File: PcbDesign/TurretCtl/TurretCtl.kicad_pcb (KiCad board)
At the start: 4 copper layers, 69.6 x 54.4 mm, 28 parts, among them J1 FLIR, J2 Stepper1, J3 Stepper2, J4 PWR

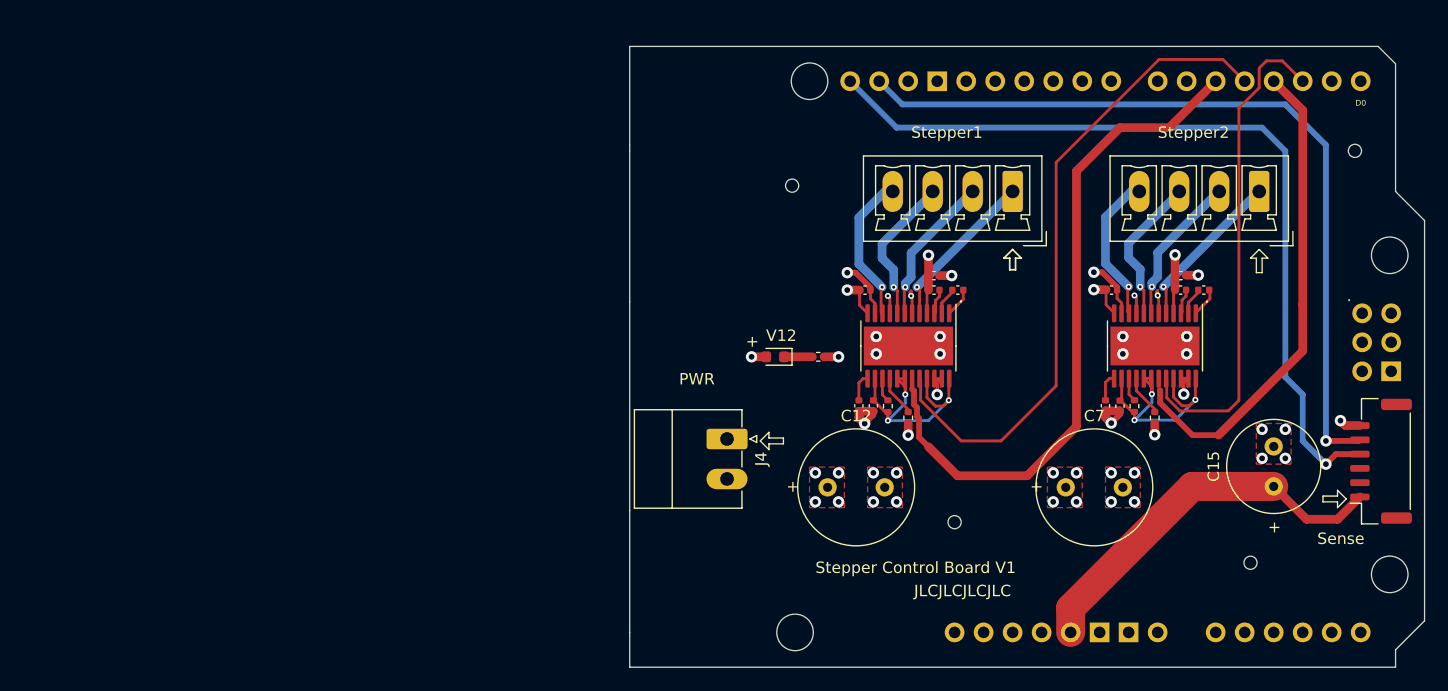
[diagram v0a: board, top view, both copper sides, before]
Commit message: Stepper Control Board V2
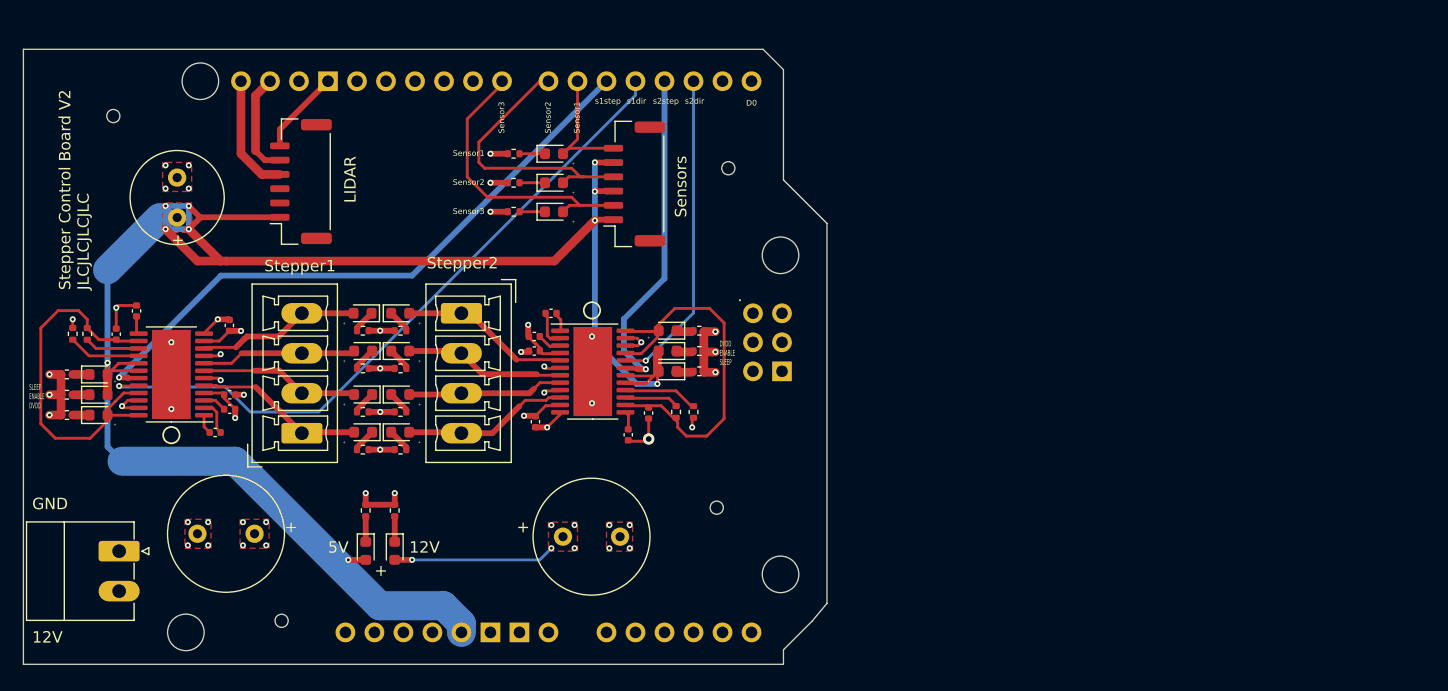
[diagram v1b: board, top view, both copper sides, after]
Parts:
- added D10: LED, LED_SMD:LED_0603_1608Metric, F.Cu at (29.2, 92.7)
- added D11: LED, LED_SMD:LED_0603_1608Metric, F.Cu at (79.0, 85.3)
- added D12: LED, LED_SMD:LED_0603_1608Metric, F.Cu at (29.2, 89.2)
- added D13: LED, LED_SMD:LED_0603_1608Metric, F.Cu at (79.0, 88.9)
- added D14: LED, LED_SMD:LED_0603_1608Metric, F.Cu at (52.6, 104.6)
- added D15: LED, LED_SMD:LED_0603_1608Metric, F.Cu at (69.1, 69.8)
- added D16: LED, LED_SMD:LED_0603_1608Metric, F.Cu at (29.2, 91.0)
- added D17: LED, LED_SMD:LED_0603_1608Metric, F.Cu at (79.0, 87.1)
- added D18: LED, LED_SMD:LED_0603_1608Metric, F.Cu at (69.1, 72.4)
- added D19: LED, LED_SMD:LED_0603_1608Metric, F.Cu at (69.1, 74.9)
- added D2: LED, LED_SMD:LED_0603_1608Metric, F.Cu at (52.3, 83.8)
- added D3: LED, LED_SMD:LED_0603_1608Metric, F.Cu at (55.6, 94.2)
- added D4: LED, LED_SMD:LED_0603_1608Metric, F.Cu at (52.3, 87.1)
- added D5: LED, LED_SMD:LED_0603_1608Metric, F.Cu at (55.6, 90.9)
- added D6: LED, LED_SMD:LED_0603_1608Metric, F.Cu at (52.3, 90.9)
- added D7: LED, LED_SMD:LED_0603_1608Metric, F.Cu at (55.6, 87.1)
- added D8: LED, LED_SMD:LED_0603_1608Metric, F.Cu at (52.3, 94.2)
- added D9: LED, LED_SMD:LED_0603_1608Metric, F.Cu at (55.6, 83.8)
- added J5: Sensors, Connector_JST:JST_GH_SM06B-GHS-TB_1x06-1MP_P1.25mm_Horizontal, F.Cu at (76.1, 72.5)
- added R10: 330, Resistor_SMD:R_0402_1005Metric, F.Cu at (52.3, 92.5)
- added R11: 330, Resistor_SMD:R_0402_1005Metric, F.Cu at (55.6, 88.6)
- added R12: 330, Resistor_SMD:R_0402_1005Metric, F.Cu at (52.3, 95.8)
- added R13: 330, Resistor_SMD:R_0402_1005Metric, F.Cu at (55.6, 85.3)
- added R14: 330, Resistor_SMD:R_0402_1005Metric, F.Cu at (26.4, 92.7)
- added R15: 330, Resistor_SMD:R_0402_1005Metric, F.Cu at (81.8, 85.3)
- added R16: 330, Resistor_SMD:R_0402_1005Metric, F.Cu at (26.4, 89.2)
- added R17: 330, Resistor_SMD:R_0402_1005Metric, F.Cu at (81.8, 88.9)
- added R18: 330, Resistor_SMD:R_0402_1005Metric, F.Cu at (52.6, 101.1)
- added R19: 330, Resistor_SMD:R_0402_1005Metric, F.Cu at (65.5, 69.8)
- added R20: 330, Resistor_SMD:R_0402_1005Metric, F.Cu at (26.4, 91.0)
- added R21: 330, Resistor_SMD:R_0402_1005Metric, F.Cu at (81.8, 87.1)
- added R22: 330, Resistor_SMD:R_0402_1005Metric, F.Cu at (65.5, 72.4)
- added R23: 330, Resistor_SMD:R_0402_1005Metric, F.Cu at (65.5, 74.9)
- added R6: 330, Resistor_SMD:R_0402_1005Metric, F.Cu at (52.3, 85.3)
- added R7: 330, Resistor_SMD:R_0402_1005Metric, F.Cu at (55.6, 95.8)
- added R8: 330, Resistor_SMD:R_0402_1005Metric, F.Cu at (52.3, 88.6)
- added R9: 330, Resistor_SMD:R_0402_1005Metric, F.Cu at (55.6, 92.5)
- R5: value 290 -> 330
- moved C15 98.9 mm to (36.1, 75.4)
- moved J1 97.7 mm to (46.9, 72.3)
- moved R1 73.5 mm to (26.9, 85.6), turned to 90 degrees
- moved C7 71.1 mm to (42.8, 103.1), turned to 180 degrees
- moved J3 70.7 mm to (61.0, 83.8), turned to -90 degrees
- moved R2 70.4 mm to (28.2, 85.6), turned to -90 degrees
- moved C8 66.6 mm to (30.7, 85.6), turned to 90 degrees
- moved C3 66.2 mm to (39.4, 94.3), turned to 180 degrees
- moved J2 65.7 mm to (47.0, 94.3), turned to 90 degrees
- moved U2 64.6 mm to (35.6, 89.2), turned to 180 degrees
- moved C9 63.8 mm to (32.5, 83.6), turned to 90 degrees
- moved C4 62.5 mm to (40.7, 92.2), turned to 180 degrees
- moved C6 62.5 mm to (40.7, 91.0)
- moved C11 57.9 mm to (67.4, 93.3), turned to -90 degrees
- moved C1 57.2 mm to (68.8, 83.8)
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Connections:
- U1 pad 17: /Stepper2/DVDD -> +5V
- U1 pad 18: /Stepper2/DVDD -> +5V
- U1 pad 25: GND -> (no net)
- U2 pad 17: /Stepper1/DVDD -> +5V
- U2 pad 18: /Stepper1/DVDD -> +5V
- U2 pad 25: GND -> (no net)
- XA1 pad D6: unconnected-(XA1-PadD6) -> D6
- XA1 pad D7: unconnected-(XA1-PadD7) -> D7
- XA1 pad D8: unconnected-(XA1-PadD8) -> D8
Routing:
- net +5V: track 33.9 -> 176.6 mm, vias 0 -> 12
- net SCL: track 72.9 -> 10.5 mm, vias 1 -> 0
- net SDA: track 70.4 -> 9.09 mm, vias 1 -> 0
- net GND: track 36.9 -> 67.2 mm, vias 36 -> 41
- net D8: track 0.00 -> 25.2 mm
- net D7: track 0.00 -> 24.4 mm
- net S2_DIR: track 43.5 -> 28.0 mm, vias 0 -> 1
- net S2_STEP: track 42.5 -> 30.4 mm, vias 0 -> 1
- net D6: track 0.00 -> 11.5 mm
- net /Stepper1/DVDD: track 23.7 -> 33.2 mm, vias 3 -> 0
- net /Stepper2/DVDD: track 23.7 -> 33.0 mm, vias 3 -> 0
- net +12V: track 21.5 -> 30.2 mm
- net S1_STEP: track 59.2 -> 56.0 mm, vias 0 -> 1
- net /Stepper2/RREF: track 3.58 -> 6.36 mm
- net /Stepper1/RREF: track 3.58 -> 6.36 mm
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- added copper zone on B.Cu, net +5V
- added copper zone on F.Cu, net +5V
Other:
- board size 69.6 x 54.4 mm -> 70.4 x 53.8 mm
- board text added: "12V"
- board text added: "5V"
- board text added: "DVDD ENABLE SLEEP"
- board text added: "GND"
- board text added: "LIDAR"
- board text added: "SLEEP ENABLE DVDD"
- board text added: "Sensor1"
- board text added: "Sensor2"
- board text added: "Sensor3"
- board text added: "Sensors"
- board text added: "Stepper Control Board V2 JLCJLCJLCJLC"
- board text added: "s1dir"
- board text added: "s1step"
- board text added: "s2dir"
- board text added: "s2step"
- board text removed: "-"
- board text removed: "A1A2B2B1"
- board text removed: "JLCJLCJLCJLC"
- board text removed: "PWR"
- board text removed: "SCL"
- board text removed: "SDA"
- board text removed: "Sense"
- board text removed: "Stepper Control Board V1"
- board text removed: "V12"
